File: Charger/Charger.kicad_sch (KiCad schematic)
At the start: 4 parts, among them J1 Bat_ballanser_conn, J2 Battery_conn, J3 Power_conn, J4 Screen_SPInCtrlnPwr_Conn

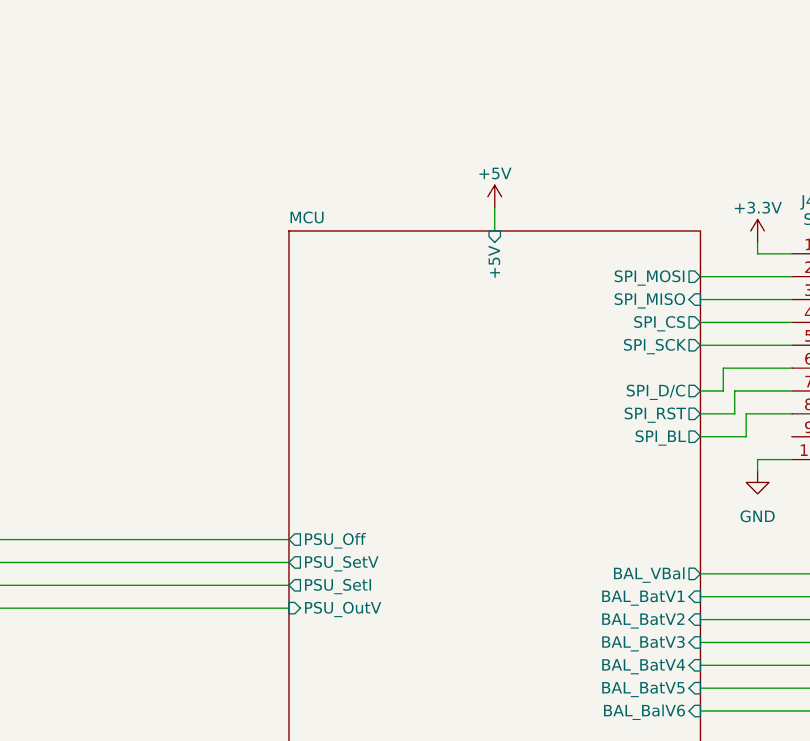
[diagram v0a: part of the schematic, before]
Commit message: Schematic trace update
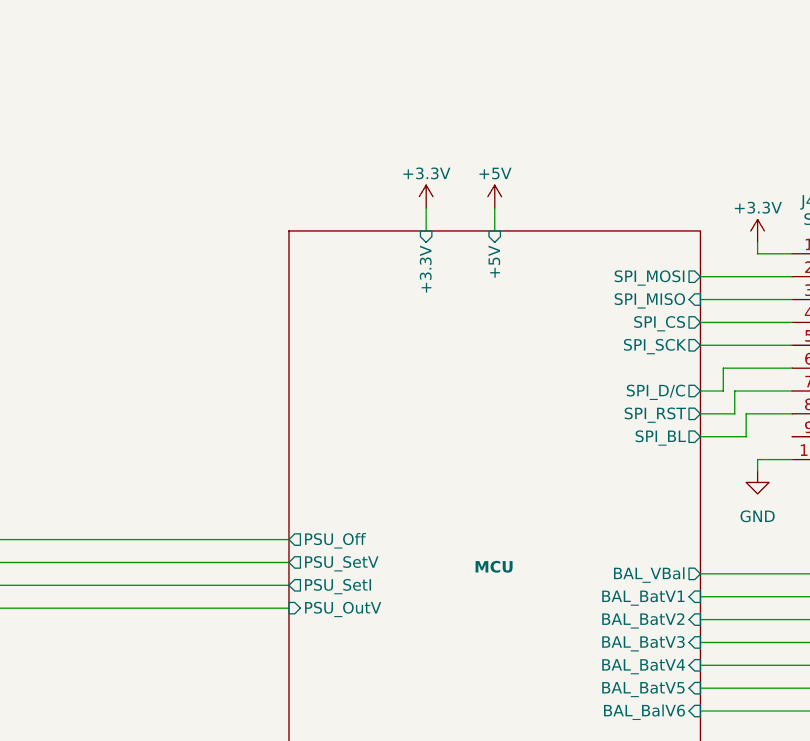
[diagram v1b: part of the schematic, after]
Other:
- sheet MCU ports: added +3.3V; removed none
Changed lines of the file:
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@@
+		)
+	)
+	(wire
+		(pts
+			(xy 134.62 30.48) (xy 134.62 33.02)
+		)
+		(stroke
+			(width 0)
+			(type default)
 		)
 	)
@@
 		)
 	)
+	(symbol
+		(lib_id "power:+3.3V")
+		(at 134.62 30.48 0)
+		(unit 1)
+		(exclude_from_sim no)
+		(in_bom yes)
+		(on_board yes)
+		(dnp no)
+		(property "Reference" "#PWR067"
+			(at 134.62 34.29 0)
+			(effects
+				(font
+					(size 1.27 1.27)
+				)
+				(hide yes)
+			)
+		)
+		(property "Value" "+3.3V"
+			(at 134.62 26.67 0)
+			(effects
+				(font
+					(size 1.27 1.27)
+				)
+			)
+		)
+		(property "Footprint" ""
+			(at 134.62 30.48 0)
+			(effects
+				(font
+					(size 1.27 1.27)
+				)
+				(hide yes)
+			)
+		)
+		(property "Datasheet" ""
+			(at 134.62 30.48 0)
+			(effects
+				(font
+					(size 1.27 1.27)
+				)
+				(hide yes)
+			)
+		)
+		(property "Description" "Power symbol creates a global label with name \"+3.3V\""
+			(at 134.62 30.48 0)
+			(effects
+				(font
+					(size 1.27 1.27)
+				)
+				(hide yes)
+			)
+		)
+		(pin "1"
+		)
+		(instances
+			(project "Charger"
+				(path "/f0501846-9b00-4ec1-8596-952177c35a04"
+					(reference "#PWR067")
+					(unit 1)
+				)
+			)
+		)
+	)
 	(sheet
 		(at 214.63 114.3)
@@
 		(at 119.38 33.02)
 		(size 45.72 73.66)
-		(fields_autoplaced yes)
 		(stroke
 			(width 0.1524)
@@
 		)
 		(property "Sheetname" "MCU"
-			(at 119.38 32.3084 0)
-			(effects
-				(font
-					(size 1.27 1.27)
+			(at 139.954 71.12 0)
+			(effects
+				(font
+					(size 1.27 1.27)
+					(bold yes)
 				)
 				(justify left bottom)
@@
 			(effects
 				(font
+					(size 1.27 1.27)
+				)
+				(justify right)
+			)
+		)
+		(pin "+3.3V" input
+			(at 134.62 33.02 90)
+			(effects
+				(font
